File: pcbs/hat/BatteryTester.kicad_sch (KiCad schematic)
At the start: 1 part, among them J1 Screw_Terminal_01x02

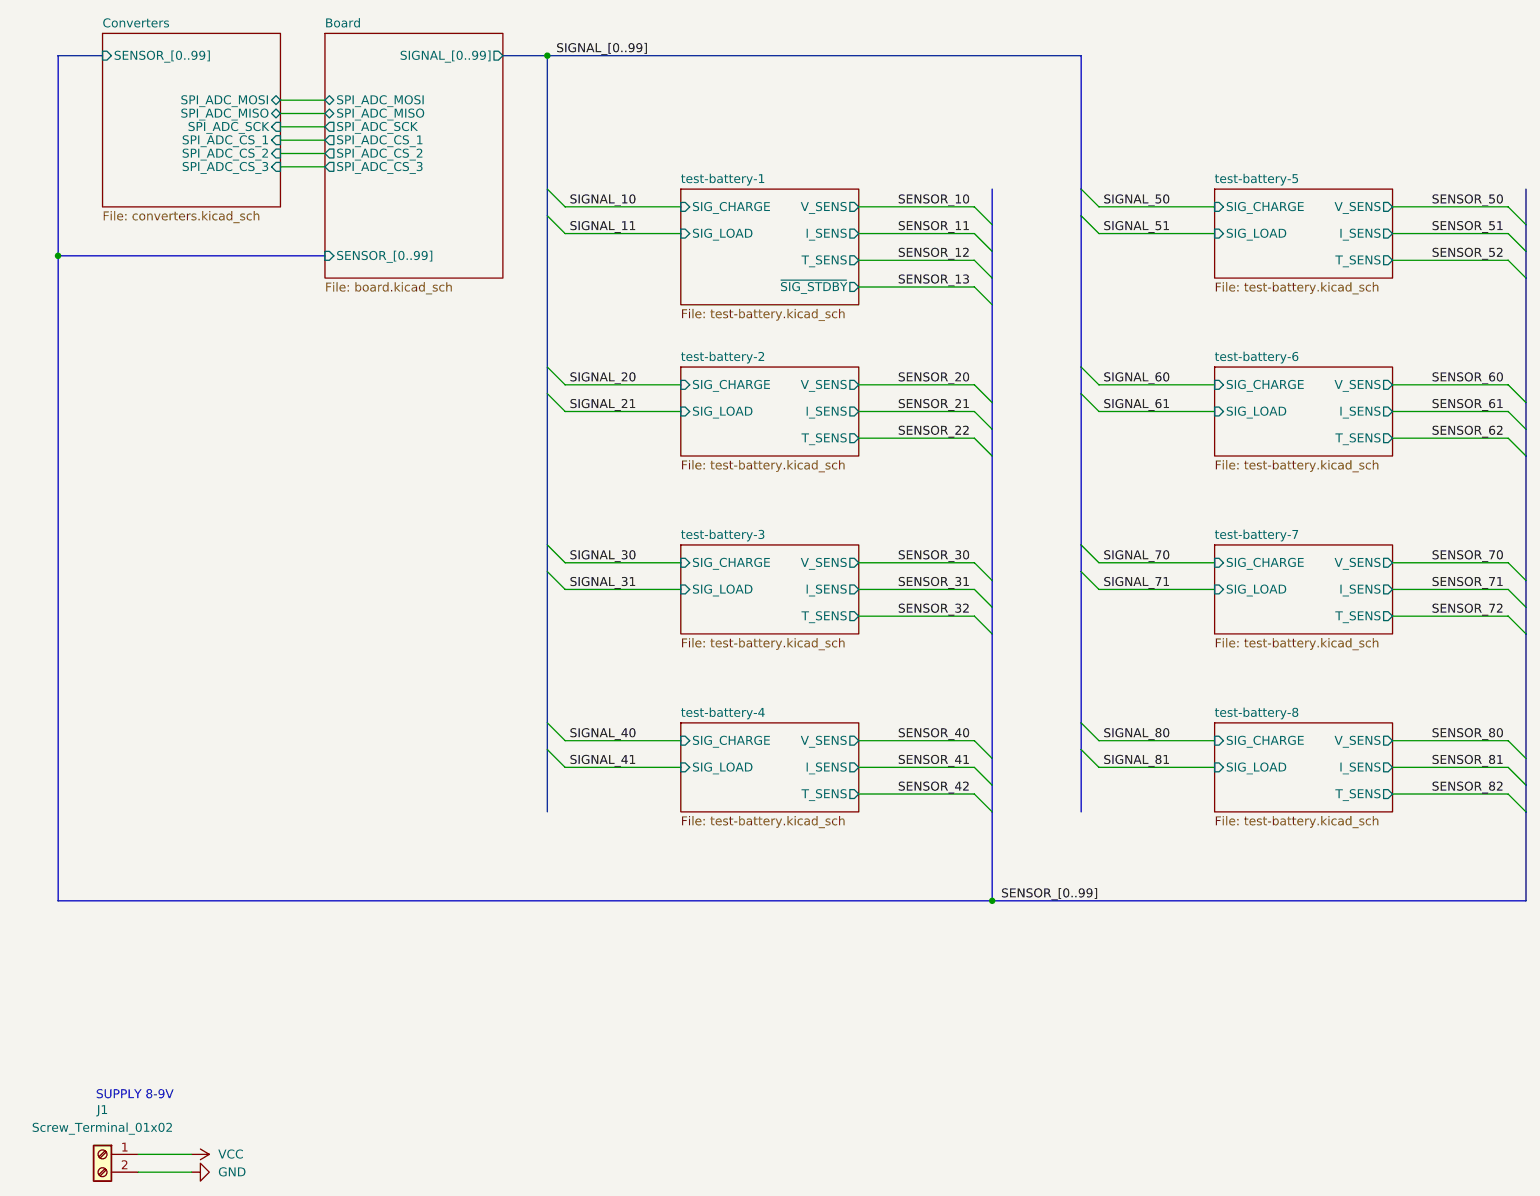
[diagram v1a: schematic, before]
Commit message: more work on charging circuit
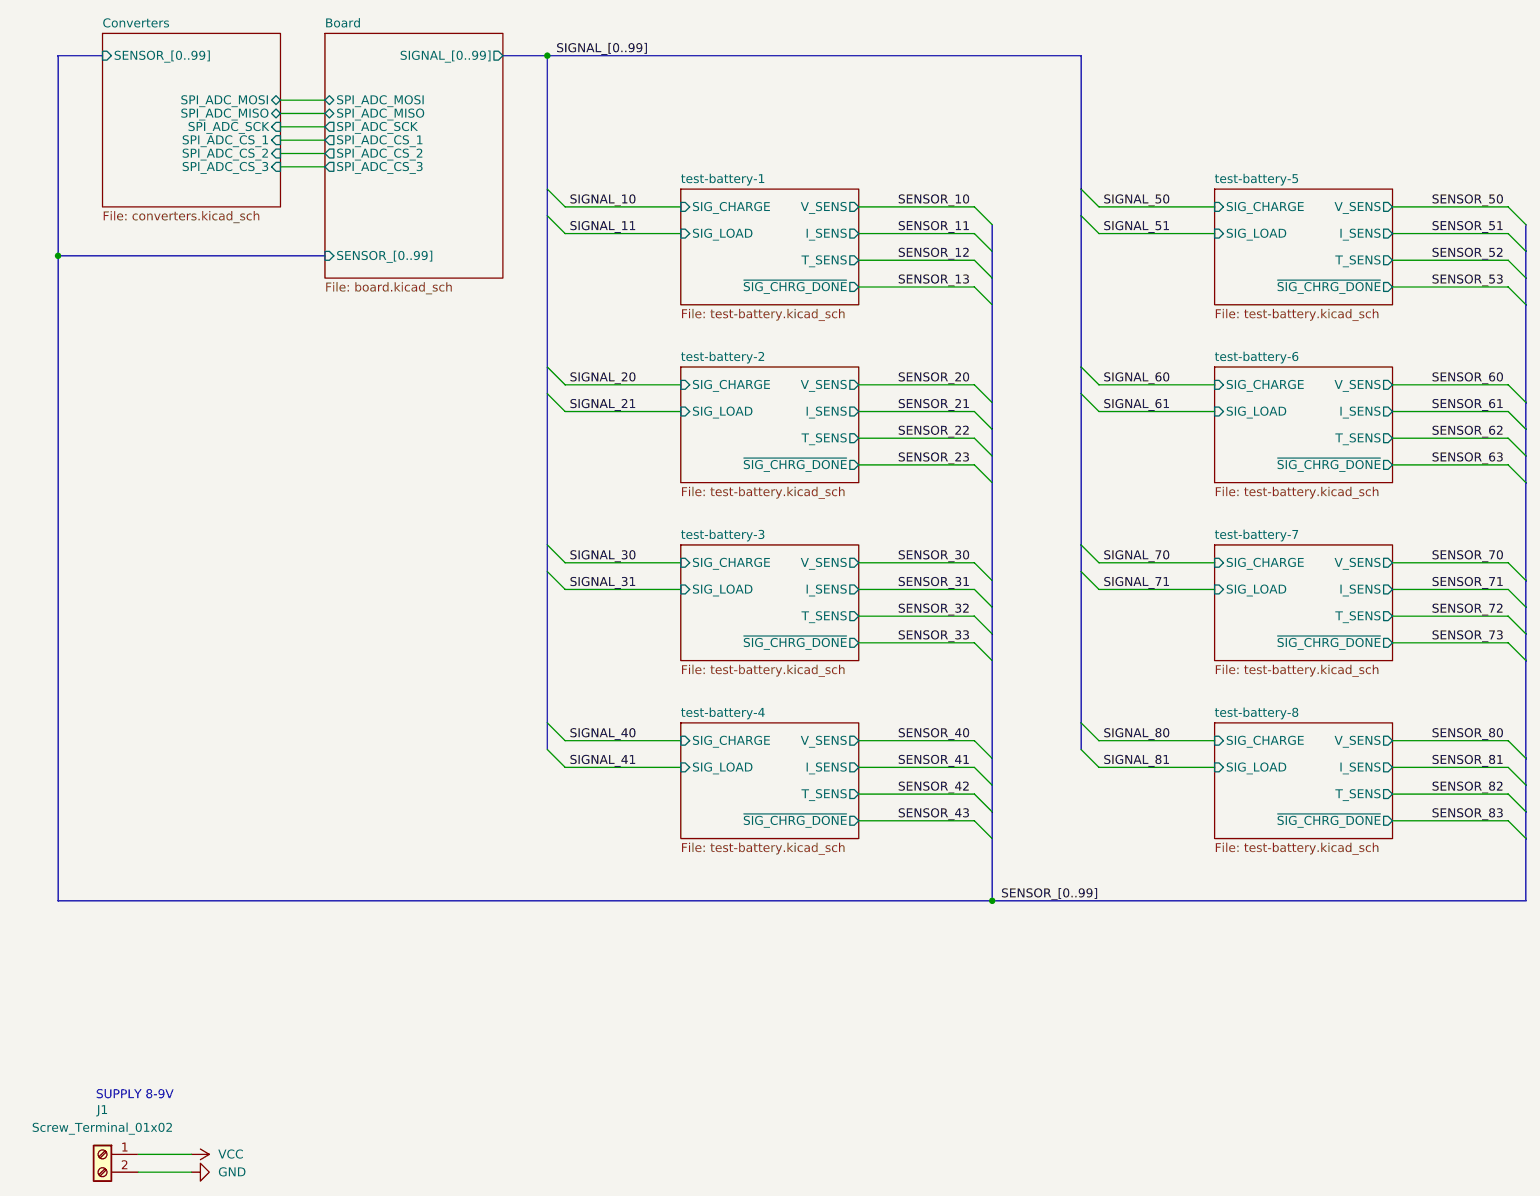
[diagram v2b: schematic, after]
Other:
- sheet test-battery-1 ports: added ~{SIG_CHRG_DONE}; removed ~{SIG_STDBY}
- sheet test-battery-2 ports: added ~{SIG_CHRG_DONE}; removed none
- sheet test-battery-3 ports: added ~{SIG_CHRG_DONE}; removed none
- sheet test-battery-4 ports: added ~{SIG_CHRG_DONE}; removed none
- sheet test-battery-5 ports: added ~{SIG_CHRG_DONE}; removed none
- sheet test-battery-6 ports: added ~{SIG_CHRG_DONE}; removed none
- sheet test-battery-7 ports: added ~{SIG_CHRG_DONE}; removed none
- sheet test-battery-8 ports: added ~{SIG_CHRG_DONE}; removed none
